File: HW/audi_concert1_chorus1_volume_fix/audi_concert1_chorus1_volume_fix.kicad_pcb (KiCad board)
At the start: 2 copper layers, 32.8 x 26.2 mm, 40 parts, among them CON1 I2C_to_TDA, CON2 USB, CON3 SPI_TO_PANEL, CON4 JLINK, U1 68HC05_PLCC, U2 AP1117-33, U3 STM32F103C8Tx, U4 MAX809, Y1 32.768kHz, Y2 8MHz

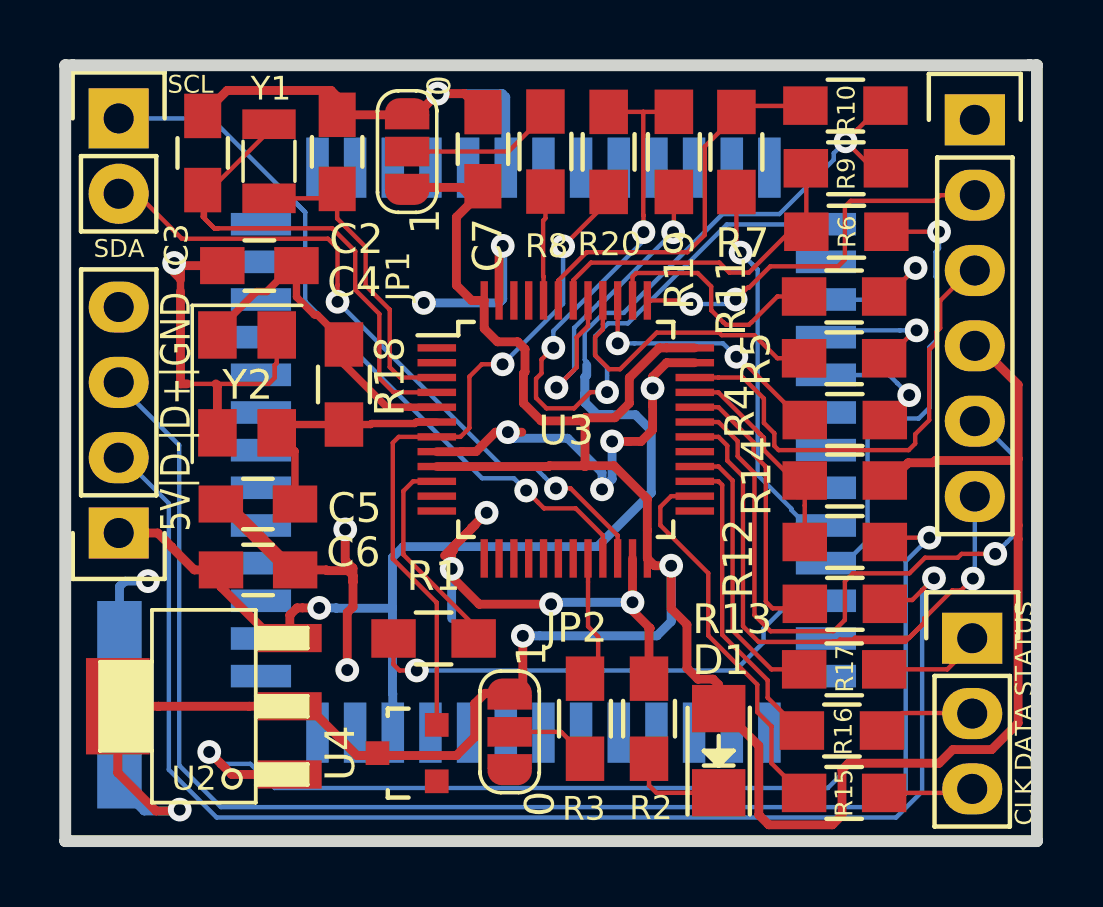
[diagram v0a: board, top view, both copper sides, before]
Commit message: HW v3
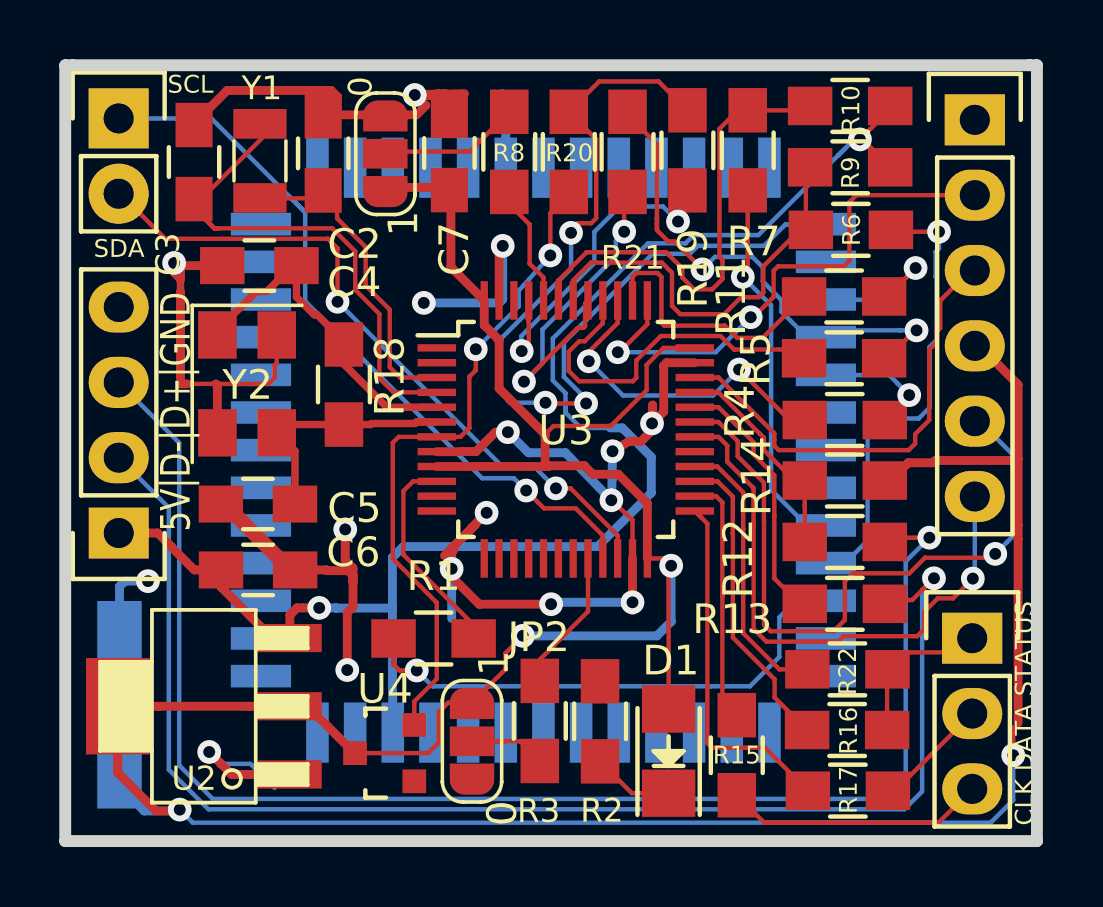
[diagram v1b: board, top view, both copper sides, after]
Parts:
- added R21: 10k, Resistors_SMD.pretty:R_0805_HandSoldering, F.Cu at (120.6, 74.0)
- added R22: 10k, Resistors_SMD.pretty:R_0805_HandSoldering, F.Cu at (128.0, 91.5)
- moved R17 4.09 mm to (128.0, 95.6)
- moved R15 3.84 mm to (124.2, 94.4), turned to 90 degrees
- moved D1 1.69 mm to (121.9, 94.2)
- moved R2 1.65 mm to (119.6, 93.2)
- moved R3 1.53 mm to (117.6, 93.2)
- moved R20 1.34 mm to (118.6, 74.0)
- moved JP2 1.31 mm to (115.3, 93.9)
- moved R8 1.22 mm to (116.6, 74.0)
- moved C7 1.14 mm to (114.6, 74.1)
- moved U4 0.76 mm to (112.4, 94.3)
- moved JP1 0.74 mm to (112.4, 74.1)
- moved C2 0.47 mm to (110.3, 74.1)
- moved R19 0.46 mm to (122.6, 74.0)
- moved C3 0.42 mm to (105.9, 74.4)
- moved R7 0.38 mm to (124.6, 74.0)
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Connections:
- CON3 pad 1: /STATUS_TO_PANEL -> /DATA_TO_PANEL
- CON3 pad 2: /DATA_TO_PANEL -> /STATUS_TO_PANEL
- U3 pad 25: (no net) -> Net-(R17-Pad2)
- U3 pad 28: Net-(R17-Pad2) -> Net-(R22-Pad2)
- U3 pad 41: Net-(R19-Pad2) -> Net-(R21-Pad2)
- U3 pad 45: (no net) -> Net-(R19-Pad2)
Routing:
- net GND: track 106.9 -> 87.2 mm
- net /DATA_FROM_MCU: track 5.27 -> 18.1 mm, vias 1 -> 2
- net 3V3: track 103.2 -> 115.7 mm, vias 3 -> 4
- net Net-(R21-Pad2): track 0.00 -> 11.6 mm, vias 0 -> 2
- net Net-(R22-Pad2): track 0.00 -> 9.41 mm
- net /CLOCK_TO_PANEL: track 3.41 -> 9.01 mm
- net /RESET_KA: track 27.5 -> 32.4 mm
- net Net-(R15-Pad2): track 13.0 -> 8.39 mm
- net /SWDCLK: track 13.7 -> 18.1 mm
- net /TX: track 23.5 -> 19.5 mm
- net Net-(R17-Pad2): track 9.48 -> 12.6 mm
- net Net-(R4-Pad1): track 8.82 -> 11.3 mm
- net Net-(R5-Pad2): track 10.1 -> 12.3 mm
- net Net-(R6-Pad1): track 11.6 -> 13.9 mm
- net /DATA_TO_PANEL: track 3.60 -> 5.59 mm
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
